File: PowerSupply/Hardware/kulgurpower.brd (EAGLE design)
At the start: 102 x 86.5 mm, 97 parts, among them X2 1727036

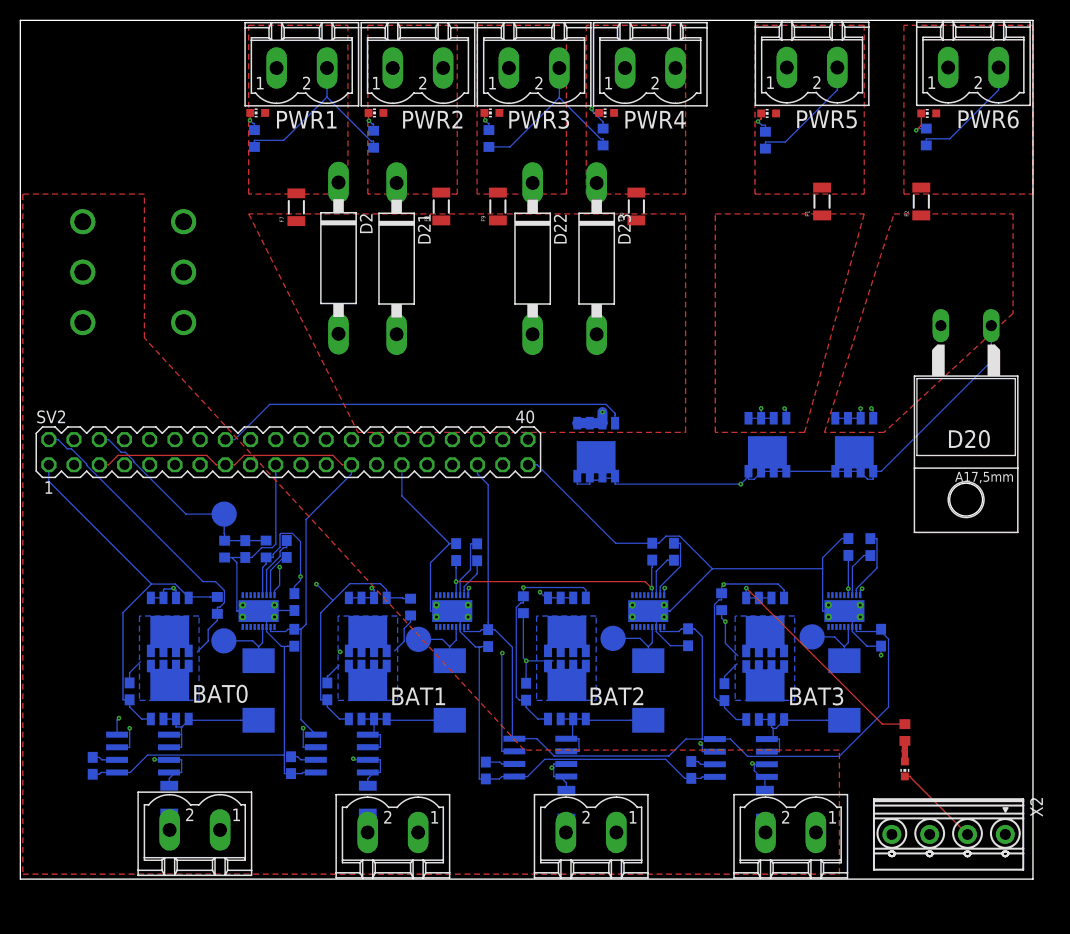
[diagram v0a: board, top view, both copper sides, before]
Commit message: Lot of changes to schematics. A lot.
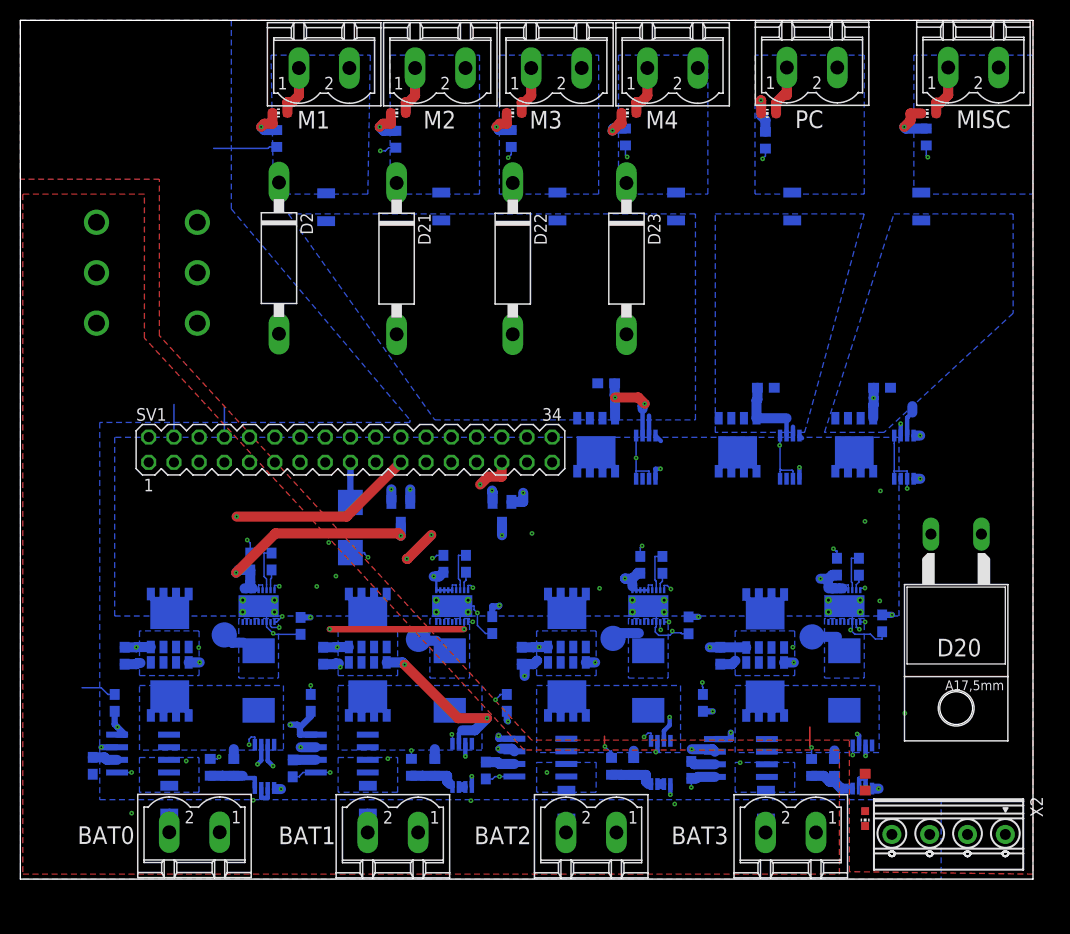
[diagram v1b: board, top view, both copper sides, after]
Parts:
- removed E-STOP: PC-6-16/2-G-10.16-1913646, phoenix-1016:PC-6-16/2-G-10.16
- removed PWR1, PWR2, PWR3, PWR4: MST2V, con-phoenix-508:MSTBV2
- removed R10, R14, R3, R5: 100k, rcl:R0603
- removed R4: 680k, rcl:R0603
- removed SV2: (no value), con-lstb:MA20-2
- removed TP13: TPB2,54, testpad:B2,54
- added C22, C23, C24, C25, C26, C27, C28: 0.1, rcl:C0603
- added D1, D3: BAT54C, diode:SOT23
- added M1, M2, M3, M4: MST2V, con-phoenix-508:MSTBV2
- added R11, R15, R17, R19: 680k, rcl:R0603
- added R13, R16, R20: 100k, rcl:R0603
- added SV1: (no value), con-lstb:MA17-2
- added U$20, U$21, U$22, U$23, U$24, U$25, U$26: MAX1614EUA, MAX1614EUA:MAX1614EUA
- added U$27: PC-6-16/2-G-10.16-1913646, phoenix-1016:PC-6-16/2-G-10.16
- C12, C19, C6: device resistor:C0603@1 -> rcl:C0603
- C2: value 0.1 -> 47uF / 10V; device rcl:C0603 -> rcl:C/6032-28R
- C9: device resistor:C0603 -> rcl:C0603
- F1, F10, F2, F3, F4, F5, F6, F7, F8, F9: value PTCSMD -> 10A FUSE 1206
- U$1, U$10, U$12, U$14, U$15, U$2, U$3, U$5, U$6, U$7, U$9: value FDMS8558S -> AON6500
- moved R18 42.9 mm to (59.5, 11.4), turned to 270 degrees
- moved D20 21.0 mm to (94.3, 28.4)
- moved C2 10.8 mm to (33.2, 35.4), turned to 90 degrees
- moved U$2 7.25 mm to (75.0, 26.0)
- moved U$5 7.25 mm to (15.0, 26.0)
- moved U$6 7.25 mm to (55.1, 26.0)
- moved U$9 7.25 mm to (35.0, 26.0)
- moved U$10 6.50 mm to (35.0, 19.2)
- moved U$12 6.50 mm to (15.0, 19.2)
- moved U$3 6.50 mm to (75.0, 19.2)
- moved U$7 6.50 mm to (55.1, 19.2)
- moved PWRLED 6.40 mm to (85.1, 6.10)
- moved R12 6.40 mm to (85.1, 9.76)
- moved C21 6.04 mm to (23.2, 32.0), turned to 90 degrees
- moved F9 6.00 mm to (54.1, 67.8), flipped to the bottom
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- renumbered PWR5 to PC, PWR6 to MISC
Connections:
- removed net EN_OUT1: SV2.16, U$1.P$4
- removed net EN_OUT2: SV2.26, U$14.P$4
- removed net EN_OUT3: SV2.36, U$15.P$4
- removed net N$18 (its old number): L2.1, TP5.TP, U$17.P$4A
- removed net N$2 (its old number): L1.1, TP8.TP, U$16.P$4A
- removed net N$23 (its old number): L3.1, TP10.TP, U$18.P$4A
- removed net N$26: L4.1, TP15.TP, U$19.P$4A
- removed net PBUS1: F10.1, F7.1, F8.1, F9.1, U$1.P$1, U$1.P$2, U$1.P$3
- removed net PBUS2: F1.1, U$14.P$1, U$14.P$2, U$14.P$3
- removed net PBUS3: F2.1, U$15.P$1, U$15.P$2, U$15.P$3
- removed net SKIP0: SV2.8
- removed net SKIP1: SV2.18
- removed net SKIP2: SV2.28
- removed net SKIP3: SV2.38
- removed net V18V_AD: C2.1, R3.2, R4.2, SV2.6, TP13.TP
- removed net VBB0: C19.1, R18.1, SV2.2, U$12.P$5, U$12.P$6, U$12.P$7, U$12.P$8, U$5.P$5, U$5.P$6, U$5.P$7, U$5.P$8
- removed net VBB1: C12.1, R14.1, SV2.12, U$10.P$5, U$10.P$6, U$10.P$7, U$10.P$8, U$9.P$5, U$9.P$6, U$9.P$7, U$9.P$8
- removed net VBB2: C6.1, R10.1, SV2.22, U$6.P$5, U$6.P$6, U$6.P$7, U$6.P$8, U$7.P$5, U$7.P$6, U$7.P$7, U$7.P$8
- removed net VBB3: C9.1, R5.1, SV2.32, U$2.P$5, U$2.P$6, U$2.P$7, U$2.P$8, U$3.P$5, U$3.P$6, U$3.P$7, U$3.P$8
- new net !OFF_0: U$20.2, U$20.3
- new net !OFF_1: U$22.2, U$22.3
- new net !OFF_2: U$21.2, U$21.3
- new net !OFF_3: U$23.2, U$23.3
- new net BAT0_G: C19.2, U$12.P$4, U$20.6, U$5.P$4
- new net BAT0_S: C19.1, U$12.P$1, U$12.P$2, U$12.P$3, U$20.7, U$5.P$1, U$5.P$2, U$5.P$3
- new net BAT1_G: C12.2, U$10.P$4, U$22.6, U$9.P$4
- new net BAT1_S: C12.1, U$10.P$1, U$10.P$2, U$10.P$3, U$22.7, U$9.P$1, U$9.P$2, U$9.P$3
- new net BAT2_G: C6.2, U$21.6, U$6.P$4, U$7.P$4
- new net BAT2_S: C6.1, U$21.7, U$6.P$1, U$6.P$2, U$6.P$3, U$7.P$1, U$7.P$2, U$7.P$3
- new net BAT3_G: C9.2, U$2.P$4, U$23.6, U$3.P$4
- new net BAT3_S: C9.1, U$2.P$1, U$2.P$2, U$2.P$3, U$23.7, U$3.P$1, U$3.P$2, U$3.P$3
- new net LBI0: R11.1, R13.2, U$20.4
- new net LBI1: R15.1, R16.2, U$22.4
- new net LBI2: R17.1, R18.2, U$21.4
- new net LBI3: R19.1, R20.2, U$23.4
- new net OUT1_EN: SV1.20, U$24.1
- new net OUT1_G: C24.2, U$1.P$4, U$24.6
- new net OUT1_S: C24.1, F10.1, F7.1, F8.1, F9.1, U$1.P$1, U$1.P$2, U$1.P$3, U$24.7
- new net OUT2_EN: SV1.22, U$25.1
- new net OUT2_G: C22.2, U$14.P$4, U$25.6
- new net OUT2_S: C22.1, F1.1, U$14.P$1, U$14.P$2, U$14.P$3, U$25.7
- new net OUT3_EN: SV1.24, U$26.1
- new net OUT3_G: C23.2, U$15.P$4, U$26.6
- new net OUT3_S: C23.1, F2.1, U$15.P$1, U$15.P$2, U$15.P$3, U$26.7
- new net VSW0: L1.1, TP8.TP, U$16.P$4A, U$16.P$4B, U$16.P$4C, U$16.P$4D, U$16.P$4E, U$16.P$4F
- new net VSW1: L2.1, TP5.TP, U$17.P$4A, U$17.P$4B, U$17.P$4C, U$17.P$4D, U$17.P$4E, U$17.P$4F
- new net VSW2: L3.1, TP10.TP, U$18.P$4A, U$18.P$4B, U$18.P$4C, U$18.P$4D, U$18.P$4E, U$18.P$4F
- new net VSW3: L4.1, TP15.TP, U$19.P$4A, U$19.P$4B, U$19.P$4C, U$19.P$4D, U$19.P$4E, U$19.P$4F
- net !SKIP0: now also SV1.2
- net !SKIP1: now also SV1.6
- net !SKIP2: now also SV1.10
- net !SKIP3: now also SV1.14
- net +19V: now also D1.3, D3.3, SV1.34, U$16.P$5B, U$16.P$5C, U$16.P$5D, U$16.P$5E, U$16.P$5F, U$17.P$5B, U$17.P$5C, U$17.P$5D, U$17.P$5E, U$17.P$5F, U$18.P$5B, U$18.P$5C, U$18.P$5D, U$18.P$5E, U$18.P$5F, U$19.P$5B, U$19.P$5C, U$19.P$5D, U$19.P$5E, U$19.P$5F; no longer R4.1
- net 5V: now also C2.+, C25.2, C26.2, C27.2, C28.2, SV1.17; no longer SV2.15, SV2.25, SV2.35, SV2.5
- net BAT-: now also U$27.P$4, U$27.P$5, U$27.P$6; no longer E-STOP.P$4
- net BAT0_EN: now also D1.1, SV1.19, U$20.1; no longer C19.2, R18.2, SV2.1, U$12.P$4, U$5.P$4
- net BAT1_EN: now also D1.2, SV1.23, U$22.1; no longer C12.2, R14.2, SV2.11, U$10.P$4, U$9.P$4
- net BAT2_EN: now also D3.1, SV1.27, U$21.1; no longer C6.2, R10.2, SV2.21, U$6.P$4, U$7.P$4
- net BAT3_EN: now also D3.2, SV1.31, U$23.1; no longer C9.2, R5.2, SV2.31, U$2.P$4, U$3.P$4
- net GND: now also C2.-, C25.1, C26.1, C27.1, C28.1, M1.2, M2.2, M3.2, M4.2, R13.1, R16.1, R18.1, R20.1, SV1.11, SV1.12, SV1.15, SV1.16, SV1.3, SV1.4, SV1.7, SV1.8, U$20.5, U$21.5, U$22.5, U$23.5, U$24.2, U$24.4, U$24.5, U$25.2, U$25.4, U$25.5, U$26.2, U$26.4, U$26.5, U$27.P$1, U$27.P$2, U$27.P$3; no longer C2.2, E-STOP.P$1, PWR1.2, PWR2.2, PWR3.2, PWR4.2, R3.1, SV2.10, SV2.19, SV2.20, SV2.29, SV2.30, SV2.39, SV2.40, SV2.9
- net IBAT0_AD: now also SV1.1; no longer SV2.7
- net IBAT1_AD: now also SV1.5; no longer SV2.17
- net IBAT2_AD: now also SV1.9; no longer SV2.27
- net IBAT3_AD: now also SV1.13; no longer SV2.37
- net PWM0: now also SV1.26; no longer SV2.4
- net PWM1: now also SV1.28; no longer SV2.14
- net PWM2: now also SV1.30; no longer SV2.24
- net PWM3: now also SV1.32; no longer SV2.34
- net PWR1: now also M1.1; no longer PWR1.1
- net PWR2: now also M2.1; no longer PWR2.1
- net PWR3: now also M3.1; no longer PWR3.1
- net PWR4: now also M4.1; no longer PWR4.1
- net V+: now also U$2.P$5, U$2.P$6, U$2.P$7, U$2.P$8, U$24.8, U$25.8, U$26.8, U$5.P$5, U$5.P$6, U$5.P$7, U$5.P$8, U$6.P$5, U$6.P$6, U$6.P$7, U$6.P$8, U$9.P$5, U$9.P$6, U$9.P$7, U$9.P$8; no longer U$10.P$1, U$10.P$2, U$10.P$3, U$12.P$1, U$12.P$2, U$12.P$3, U$3.P$1, U$3.P$2, U$3.P$3, U$7.P$1, U$7.P$2, U$7.P$3
- net VBAT0: now also SV1.21; no longer SV2.3
- net VBAT0_X: now also R11.2, U$12.P$5, U$12.P$6, U$12.P$7, U$12.P$8, U$20.8; no longer U$5.P$1, U$5.P$2, U$5.P$3
- net VBAT1: now also SV1.25; no longer SV2.13
- net VBAT1_X: now also R15.2, U$10.P$5, U$10.P$6, U$10.P$7, U$10.P$8, U$22.8; no longer U$9.P$1, U$9.P$2, U$9.P$3
- net VBAT2: now also SV1.29; no longer SV2.23
- net VBAT2_X: now also R17.2, U$21.8, U$7.P$5, U$7.P$6, U$7.P$7, U$7.P$8; no longer U$6.P$1, U$6.P$2, U$6.P$3
- net VBAT3: now also SV1.33; no longer SV2.33
- net VBAT3_X: now also R19.2, U$23.8, U$3.P$5, U$3.P$6, U$3.P$7, U$3.P$8; no longer U$2.P$1, U$2.P$2, U$2.P$3
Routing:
- net GND: track 507.1 -> 178.0 mm, vias 1 -> 36
- net V+: track 160.9 -> 48.6 mm, vias 5 -> 4
- net !SKIP3: track 0.00 -> 66.0 mm, vias 0 -> 1
- net OUT3_EN: track 0.00 -> 53.4 mm, vias 0 -> 1
- net !SKIP2: track 0.00 -> 52.0 mm, vias 0 -> 2
- net +19V: track 113.8 -> 160.7 mm, vias 4 -> 6
- net EN_OUT2: track 46.0 -> 0.00 mm, vias 1 -> 0
- net VBB3: track 45.5 -> 0.00 mm, vias 1 -> 0
- net OUT2_EN: track 0.00 -> 44.8 mm, vias 0 -> 1
- net VBB2: track 43.7 -> 0.00 mm, vias 1 -> 0
- net EN_OUT3: track 42.4 -> 0.00 mm, vias 1 -> 0
- net EN_OUT1: track 42.1 -> 0.00 mm
- net VBB1: track 38.6 -> 0.00 mm, vias 1 -> 0
- net 5V: track 203.0 -> 166.1 mm, vias 1 -> 15
- net !SKIP1: track 0.00 -> 35.9 mm, vias 0 -> 1
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- added copper zone on layer 16, net BAT0_S
- added copper zone on layer 16, net BAT1_S
- added copper zone on layer 16, net BAT2_S
- added copper zone on layer 16, net BAT3_S
- added copper zone on layer 1, net GND
- added copper zone on layer 16, net GND
- added copper zone on layer 16, net OUT1_S
- added copper zone on layer 16, net OUT2_S
- added copper zone on layer 16, net OUT3_S
- added copper zone on layer 16, net PWR1
- added copper zone on layer 16, net PWR2
- added copper zone on layer 16, net PWR3
- added copper zone on layer 16, net PWR4
- added copper zone on layer 16, net PWR5
- added copper zone on layer 16, net PWR6
- added copper zone on layer 16, net V+
- added copper zone on layer 16, net VBAT0
- added copper zone on layer 16, net VBAT0_X
- added copper zone on layer 16, net VBAT1
- added copper zone on layer 16, net VBAT1_X
- added copper zone on layer 16, net VBAT2
- added copper zone on layer 16, net VBAT2_X
- added copper zone on layer 16, net VBAT3
- added copper zone on layer 16, net VBAT3_X
- added copper zone on layer 16, net VSW0
- added copper zone on layer 16, net VSW1
- added copper zone on layer 16, net VSW2
- added copper zone on layer 16, net VSW3
- removed copper zone on layer 1, net PBUS1
- removed copper zone on layer 1, net PBUS2
- removed copper zone on layer 1, net PBUS3
- removed copper zone on layer 1, net PWR1
- removed copper zone on layer 1, net PWR2
- removed copper zone on layer 1, net PWR3
- removed copper zone on layer 1, net PWR4
- removed copper zone on layer 1, net PWR5
- removed copper zone on layer 1, net PWR6
- removed copper zone on layer 16, net VBB0
- removed copper zone on layer 16, net VBB1
- removed copper zone on layer 16, net VBB2
- removed copper zone on layer 16, net VBB3

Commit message: lot of work done on schematics
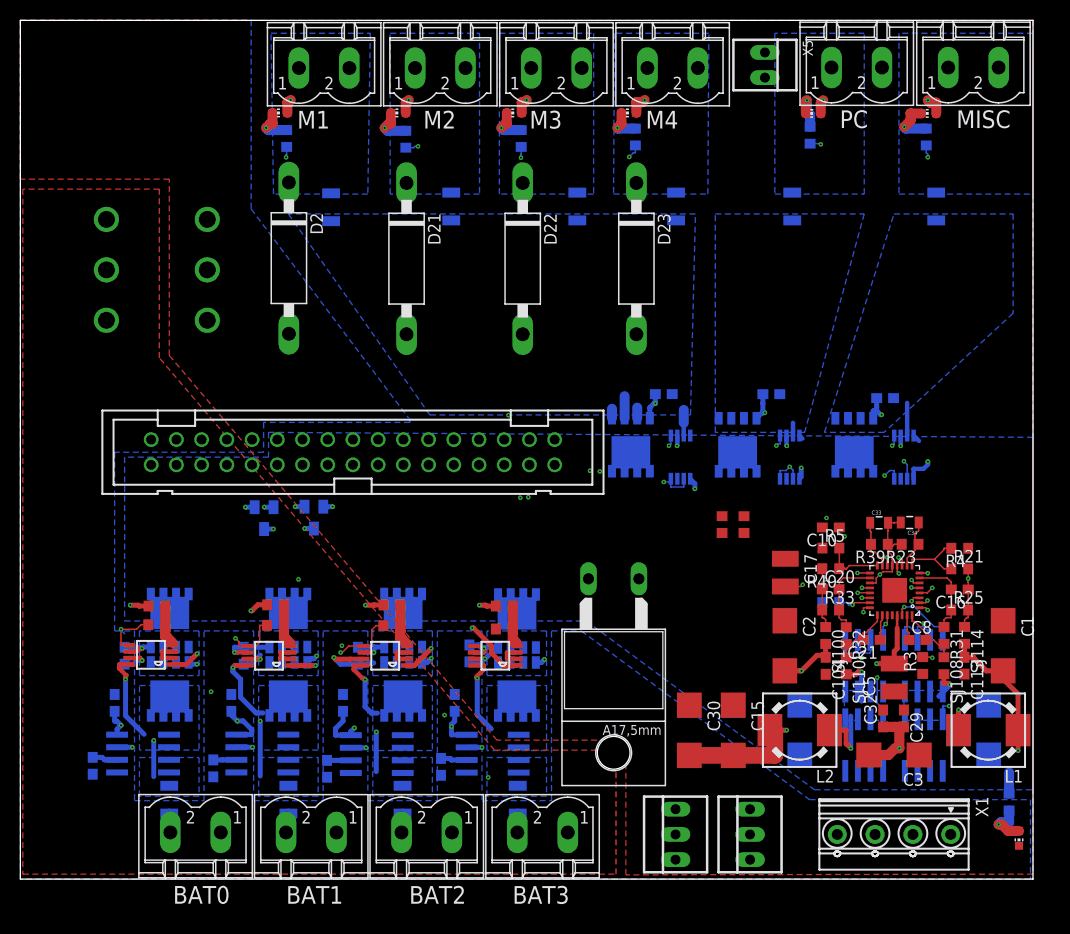
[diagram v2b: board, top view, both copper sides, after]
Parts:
- removed L3, L4: 4,7uH, inductors:DR73
- removed SV1: (no value), con-lstb:MA17-2
- removed TP10, TP15, TP5, TP8: TPB2,54, testpad:B2,54
- removed U$16, U$18, U$19: CSD97374Q4M, CSD97374Q4M:CSD97374Q4M
- added C104, C113, C32: 220n, rcl:C0603
- added C29: 0,1u, rcl:C0603
- added C30: (no value), rcl:C/6032-28R
- added C33, C34: 100pF, SparkFun:0805
- added R10, R14, R25, R33: 100k, rcl:R0603
- added R21: 120k, rcl:R0603
- added R23: 18k, rcl:R0603
- added R3: 300k, rcl:R0603
- added R31, R32: 3k16, rcl:R0603
- added R39, R4, R5: 30k, rcl:R0603
- added R40: 270k, rcl:R0603
- added SJ100, SJ104, SJ108, SJ110, SJ114: 0R, rcl:R0603
- added U$105, U$106, U$107, U$108: IRF8252, tonu:SO8
- added X1: 1727036, con-phoenix-3.81:1727036
- added X3, X4: 22-23-2031, con-molex:22-23-2031
- added X5: 22-23-2021, con-molex:22-23-2021
- C1, C13, C14, C15, C3: value 0.1 -> (none); device rcl:C0603 -> rcl:C/6032-28R
- C10: value 0.1 -> 220n
- C16, C20, C21, C8: value 0.1 -> 0,1u
- C17: value 0.1 -> 10uF/6.3V; device rcl:C0603 -> rcl:C1210
- C2: value 47uF / 10V -> (none)
- C5: value 0.1 -> 10u; device rcl:C0603 -> rcl:C1210
- U$17: value CSD97374Q4M -> TPS51222RTVT; device CSD97374Q4M:CSD97374Q4M -> tps51222:QFN-32
- X2: value 1727036 -> 2534-; device con-phoenix-3.81:1727036 -> con-3m:PAK100/2500-34
- moved C1 74.2 mm to (99.0, 23.5), flipped to the top, turned to 270 degrees
- moved L1 73.7 mm to (97.5, 15.0), flipped to the top, turned to 180 degrees
- moved X2 71.3 mm to (33.5, 43.0), turned to 0 degrees
- moved C21 63.1 mm to (85.7, 24.1), flipped to the top, turned to 180 degrees
- moved C3 61.2 mm to (88.0, 12.5), flipped to the top, turned to 180 degrees
- moved C5 46.8 mm to (88.0, 20.3), flipped to the top
- moved C8 46.1 mm to (90.4, 24.1), flipped to the top, turned to 0 degrees
- moved C2 45.4 mm to (77.0, 23.5), flipped to the top, turned to 270 degrees
- moved U$17 44.6 mm to (88.1, 29.1), flipped to the top, turned to 90 degrees
- moved C13 38.8 mm to (97.5, 15.0)
- moved U$23 38.6 mm to (47.8, 22.5), flipped to the top, turned to 90 degrees
- moved R19 37.0 mm to (48.8, 27.5), flipped to the top, turned to 180 degrees
- moved L2 35.6 mm to (78.5, 15.0), flipped to the top, turned to 180 degrees
- moved C10 35.5 mm to (81.6, 35.4), flipped to the top, turned to 180 degrees
- moved D20 34.8 mm to (59.8, 23.9)
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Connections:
- removed net !SKIP0: SV1.2, U$16.P$1
- removed net !SKIP1: SV1.6, U$17.P$1
- removed net !SKIP2: SV1.10, U$18.P$1
- removed net !SKIP3: SV1.14, U$19.P$1
- removed net N$2: C8.1, U$17.P$7
- removed net N$20: C17.2, U$19.P$6
- removed net N$22: C1.2, U$16.P$6
- removed net N$23: C14.1, U$18.P$7
- removed net N$3: C8.2, U$17.P$6
- removed net PWM0: SV1.26, U$16.P$8
- removed net PWM1: SV1.28, U$17.P$8
- removed net PWM2: SV1.30, U$18.P$8
- removed net PWM3: SV1.32, U$19.P$8
- removed net VSW0: L1.1, TP8.TP, U$16.P$4A, U$16.P$4B, U$16.P$4C, U$16.P$4D, U$16.P$4E, U$16.P$4F
- removed net VSW1: L2.1, TP5.TP, U$17.P$4A, U$17.P$4B, U$17.P$4C, U$17.P$4D, U$17.P$4E, U$17.P$4F
- removed net VSW2: L3.1, TP10.TP, U$18.P$4A, U$18.P$4B, U$18.P$4C, U$18.P$4D, U$18.P$4E, U$18.P$4F
- removed net VSW3: L4.1, TP15.TP, U$19.P$4A, U$19.P$4B, U$19.P$4C, U$19.P$4D, U$19.P$4E, U$19.P$4F
- new net +5V: C1.+, C113.1, C13.+, L1.1, SJ114.2, X1.1
- new net COMP1: C34.1, R23.1, U$17.P$10
- new net COMP2: C33.1, R39.2, U$17.P$15
- new net COMPUTER_PWR: X2.28, X5.2
- new net CSN1: C16.1, R21.2, R25.2, SJ114.1, U$17.P$2, U$17.P$8
- new net CSN2: C20.1, R33.1, R40.2, SJ100.1, U$17.P$17
- new net CSP1: C16.2, R25.1, R31.1, U$17.P$7
- new net CSP2: C20.2, R32.1, R33.2, U$17.P$18
- new net DRVH1: U$105.4, U$17.P$1
- new net DRVH2: U$108.4, U$17.P$24
- new net DRVL1: U$106.4, U$17.P$30
- new net DRVL2: U$107.4, U$17.P$27
- new net ENABLE_PWR: U$17.P$12, X2.30
- new net IMON1: U$17.P$11, X2.27
- new net IMON2: U$17.P$14, X2.29
- new net N$29: C8.1, U$17.P$31
- new net N$30: C21.1, U$17.P$26
- new net OUT4_EN: U$17.P$4, X2.24
- new net OUT5_EN: U$17.P$21, X2.26
- new net PGOOD1: R10.2, U$17.P$5, X2.31
- new net PGOOD2: R14.2, U$17.P$20, X2.33
- new net PWM_A: X2.34, X3.3
- new net PWM_B: X2.32, X4.3
- new net SERVO: C104.1, C14.+, C15.+, C2.+, C30.+, L2.2, SJ100.2, X1.3, X3.2, X4.2
- new net SW1: C8.2, R31.2, SJ108.1, U$17.P$32
- new net SW2: C21.2, R32.2, SJ110.1, U$17.P$25
- new net VIN: SJ104.1, U$17.P$23
- new net VREF2: C10.1, C33.2, C34.2, R23.2, R39.1, U$17.P$13, U$17.P$19, U$17.P$6
- new net VREG3: C17.2, R10.1, R14.1, U$17.P$22
- new net X1: L1.2, SJ108.2, U$105.1, U$105.2, U$105.3, U$106.5, U$106.6, U$106.7, U$106.8
- new net X2: L2.1, SJ110.2, U$107.5, U$107.6, U$107.7, U$107.8, U$108.1, U$108.2, U$108.3
- net +19V: now also X2.14, X2.16; no longer C13.1, C16.1, C21.1, C5.1, SV1.34, U$16.P$5A, U$16.P$5B, U$16.P$5C, U$16.P$5D, U$16.P$5E, U$16.P$5F, U$17.P$5A, U$17.P$5B, U$17.P$5C, U$17.P$5D, U$17.P$5E, U$17.P$5F, U$18.P$5A, U$18.P$5B, U$18.P$5C, U$18.P$5D, U$18.P$5E, U$18.P$5F, U$19.P$5A, U$19.P$5B, U$19.P$5C, U$19.P$5D, U$19.P$5E, U$19.P$5F, X2.1
- net 5V: now also C5.2, U$17.P$29; no longer C10.1, C15.1, C2.+, C20.1, C3.1, SV1.17, U$16.P$2, U$17.P$2, U$18.P$2, U$19.P$2
- net BAT0_EN: now also X2.9; no longer SV1.19
- net BAT1_EN: now also X2.11; no longer SV1.23
- net BAT2_EN: now also X2.13; no longer SV1.27
- net BAT3_EN: now also X2.15; no longer SV1.31
- net GND: now also C1.-, C104.2, C113.2, C13.-, C14.-, C15.-, C17.1, C29.1, C3.-, C30.-, C32.2, C5.1, R3.1, R4.1, R5.1, U$106.1, U$106.2, U$106.3, U$107.1, U$107.2, U$107.3, U$17.P$28, U$17.P$33, X1.2, X1.4, X2.10, X2.17, X3.1, X4.1, X5.1; no longer C13.2, C15.2, C16.2, C20.2, C21.2, C3.2, C5.2, SV1.11, SV1.12, SV1.15, SV1.16, SV1.3, SV1.4, SV1.7, SV1.8, U$16.P$3, U$16.PAD@1, U$17.P$3, U$17.PAD@1, U$18.P$3, U$18.PAD@1, U$19.P$3, U$19.PAD@1, X2.2
- net IBAT0_AD: now also X2.19; no longer SV1.1
- net IBAT1_AD: now also X2.21; no longer SV1.5
- net IBAT2_AD: now also X2.23; no longer SV1.9
- net IBAT3_AD: now also X2.25; no longer SV1.13
- net N$18: now also R40.1, R5.2, U$17.P$16; no longer C17.1, U$19.P$7
- net N$24: now also R3.2, U$17.P$3; no longer C14.2, U$18.P$6
- net N$5: now also R21.1, R4.2, U$17.P$9; no longer C1.1, U$16.P$7
- net OUT1_EN: now also X2.18; no longer SV1.20
- net OUT2_EN: now also X2.20; no longer SV1.22
- net OUT3_EN: now also X2.22; no longer SV1.24
- net V+: now also C29.2, C3.+, C32.1, SJ104.2, U$105.5, U$105.6, U$105.7, U$105.8, U$108.5, U$108.6, U$108.7, U$108.8, X2.12
- net VBAT0: now also X2.1, X2.2; no longer SV1.21
- net VBAT0_X: no longer L1.2
- net VBAT1: now also X2.3, X2.4; no longer SV1.25
- net VBAT1_X: no longer L2.2
- net VBAT2: now also X2.5, X2.6; no longer SV1.29
- net VBAT2_X: no longer L3.2
- net VBAT3: now also X2.7, X2.8; no longer SV1.33
- net VBAT3_X: no longer L4.2
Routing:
- net +19V: track 160.7 -> 16.8 mm, vias 6 -> 2
- net GND: track 178.0 -> 53.4 mm, vias 36 -> 18
- net !SKIP3: track 66.0 -> 0.00 mm, vias 1 -> 0
- net 5V: track 166.1 -> 103.5 mm, vias 15 -> 5
- net OUT4_EN: track 0.00 -> 59.5 mm, vias 0 -> 1
- net SERVO: track 0.00 -> 56.1 mm, vias 0 -> 2
- net !SKIP2: track 52.0 -> 0.00 mm, vias 2 -> 0
- net OUT5_EN: track 0.00 -> 48.6 mm, vias 0 -> 2
- net COMPUTER_PWR: track 0.00 -> 48.4 mm
- net IMON1: track 0.00 -> 47.6 mm, vias 0 -> 2
- net PGOOD1: track 0.00 -> 46.5 mm, vias 0 -> 2
- net ENABLE_PWR: track 0.00 -> 46.2 mm, vias 0 -> 1
- net PWM_A: track 0.00 -> 45.4 mm
- net PWM3: track 45.0 -> 0.00 mm, vias 2 -> 0
- net IMON2: track 0.00 -> 43.9 mm, vias 0 -> 2
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- added copper zone on layer 16, net X1
- added copper zone on layer 16, net X2
- removed copper zone on layer 16, net VSW0
- removed copper zone on layer 16, net VSW1
- removed copper zone on layer 16, net VSW2
- removed copper zone on layer 16, net VSW3

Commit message: More work on electronics
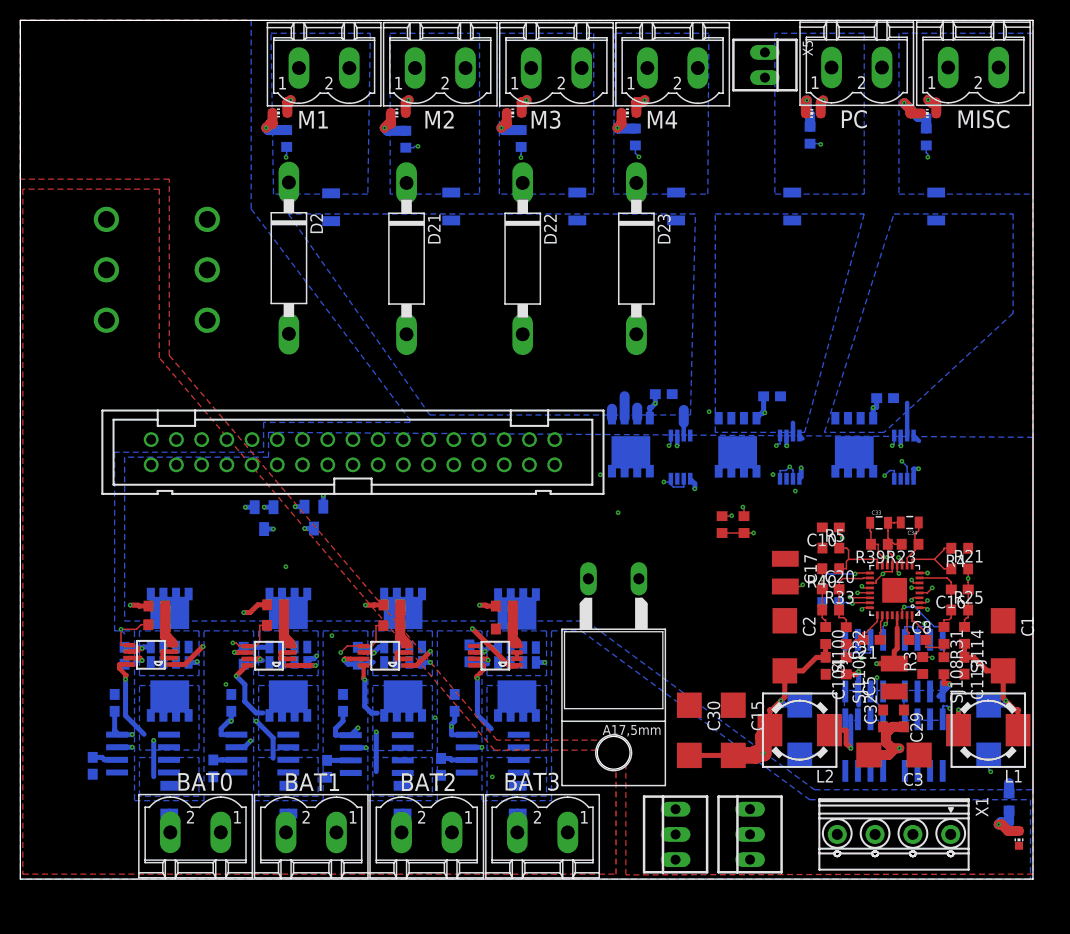
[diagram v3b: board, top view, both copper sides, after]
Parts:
- moved C22 0.24 mm to (75.7, 48.6)
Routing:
- net VREG3: track 9.13 -> 19.6 mm, vias 2 -> 3
- net +5V: track 26.1 -> 30.6 mm
- net GND: track 53.4 -> 57.1 mm, vias 18 -> 20
- net SERVO: track 56.1 -> 53.3 mm
- net VBAT1: track 38.5 -> 36.1 mm
- net BAT2_S: track 7.43 -> 5.24 mm
- net !OFF_3: track 2.66 -> 0.65 mm
- net OUT5_EN: track 48.6 -> 50.2 mm, vias 2 -> 1
- net VBAT2_X: track 16.6 -> 15.1 mm
- net N$17: track 5.00 -> 6.38 mm
- net OUT3_EN: track 57.9 -> 56.8 mm
- net PGOOD1: track 46.5 -> 45.4 mm, vias 2 -> 3
- net PGOOD2: track 36.9 -> 37.9 mm, vias 2 -> 3
- net N$18: track 6.43 -> 7.24 mm
- net V+: track 10.9 -> 10.3 mm
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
